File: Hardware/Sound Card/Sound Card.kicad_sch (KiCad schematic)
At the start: 35 parts, among them J1 ICSP, J2 6502 Card Edge, J3 Conn_02x08_Odd_Even, J4 PORT A, J5 3.5mm TRS, U1 ATmega328P-A, U2 74HC245, U3 74HC245, U4 74HC138, U5 AY-3-8912, U6 LM386, X1 2 MHz, Y1 16MHz

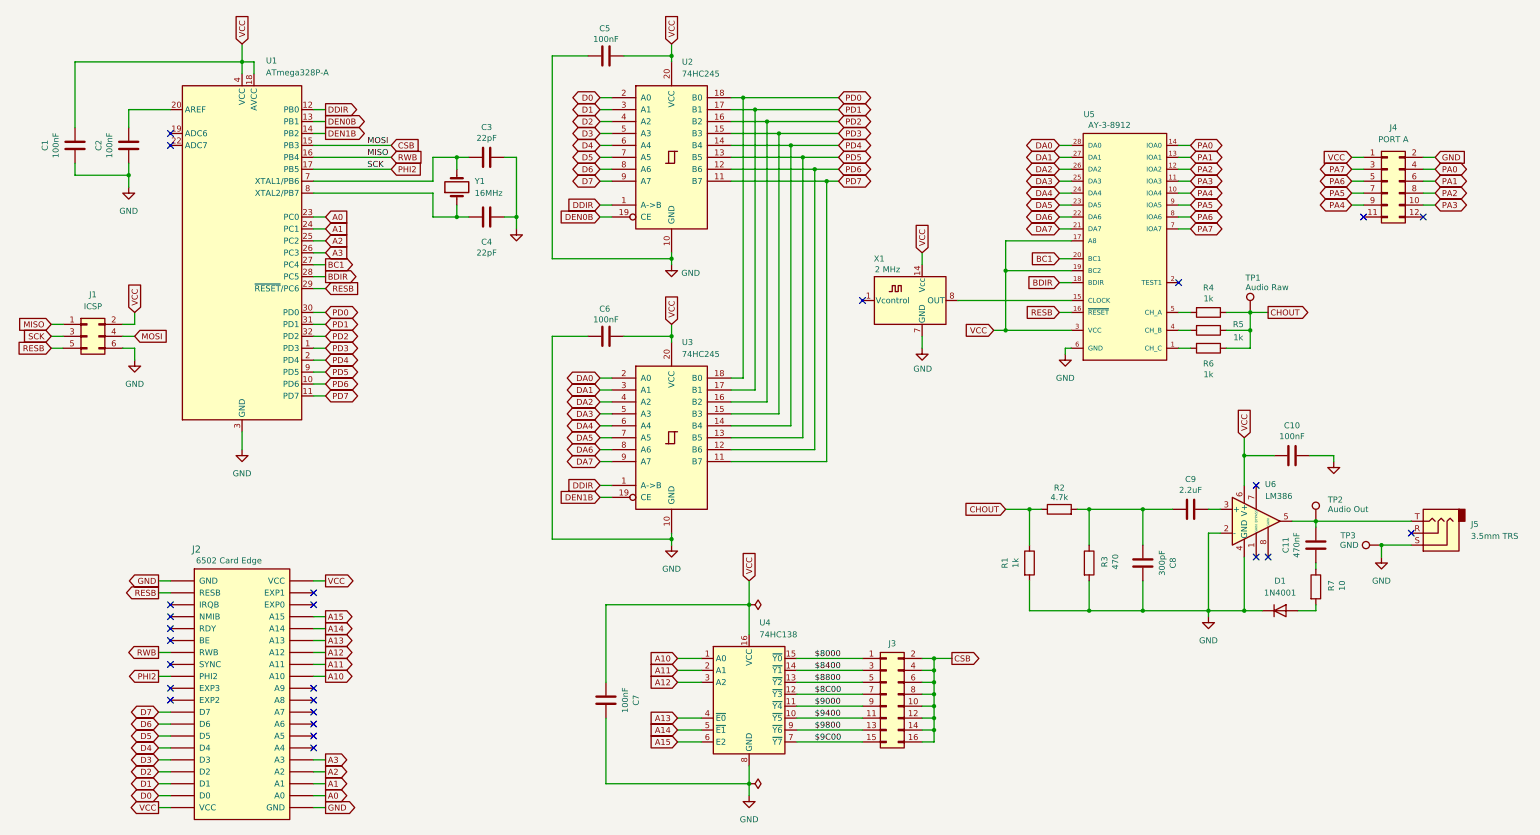
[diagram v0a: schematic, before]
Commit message: Add Wozmon
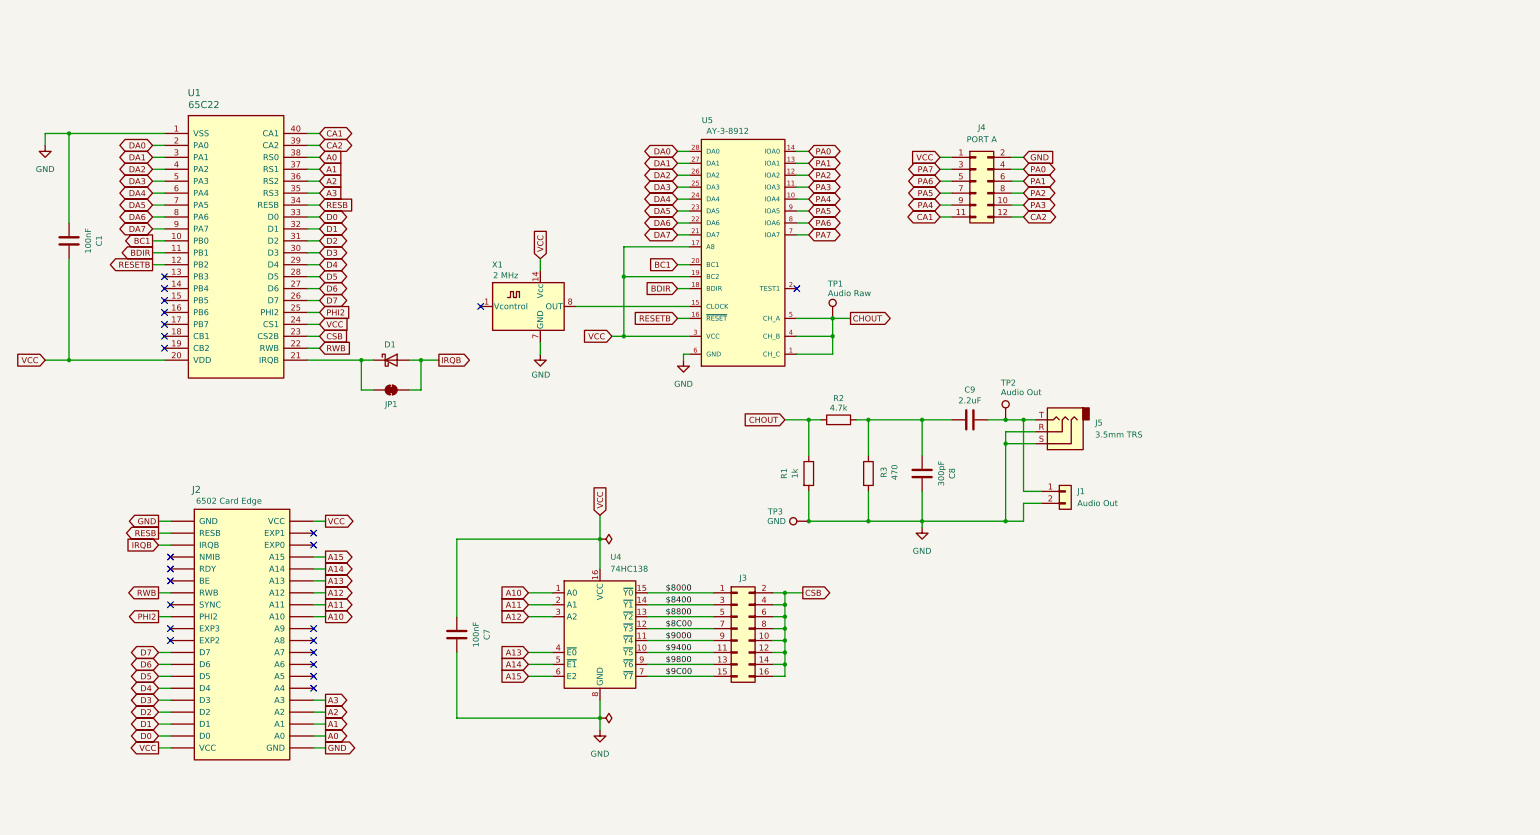
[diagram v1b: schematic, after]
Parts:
- removed C10, C2, C5, C6: 100nF, Capacitor_SMD:C_0805_2012Metric, symbol Device:C
- removed C11: 470nF, Capacitor_SMD:C_0805_2012Metric, symbol Device:C
- removed C3, C4: 22pF, Capacitor_SMD:C_0805_2012Metric, symbol Device:C
- removed D1: 1N4001, Diode_SMD:D_SMA, symbol Diode:1N4001
- removed J1: ICSP, Connector_PinHeader_2.54mm:PinHeader_2x03_P2.54mm_Vertical, symbol Connector_Generic:Conn_02x03_Odd_Even
- removed R4, R5, R6: 1k, Resistor_SMD:R_0805_2012Metric, symbol Device:R
- removed R7: 10, Resistor_SMD:R_0805_2012Metric, symbol Device:R
- removed U1: ATmega328P-A, Package_QFP:TQFP-32_7x7mm_P0.8mm, symbol MCU_Microchip_ATmega:ATmega328P-A
- removed U2, U3: 74HC245, Package_SO:SOIC-20W_7.5x12.8mm_P1.27mm, symbol 74xx:74HC245
- removed U6: LM386, Package_SO:SOP-8_3.76x4.96mm_P1.27mm, symbol Amplifier_Audio:LM386
- removed Y1: 16MHz, Crystal:Crystal_HC49-U_Vertical, symbol Device:Crystal
- added D1: D_Schottky, Diode_THT:D_DO-35_SOD27_P7.62mm_Horizontal, symbol Device:D_Schottky
- added J1: Audio Out, Connector_JST:JST_XH_B2B-XH-A_1x02_P2.50mm_Vertical, symbol Connector_Generic:Conn_01x02
- added JP1: SolderJumper_2_Bridged, Jumper:SolderJumper-2_P1.3mm_Bridged_RoundedPad1.0x1.5mm, symbol Jumper:SolderJumper_2_Bridged
- added U1: 65C22, Package_DIP:DIP-40_W15.24mm_Socket_LongPads, symbol 6502 Parts:65C22
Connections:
- net A0: now also U1.38 (RS0)
- net A1: now also U1.37 (RS1)
- net A2: now also U1.36 (RS2)
- net A3: now also U1.35 (RS3)
- net BC1: now also U1.10 (PB0)
- net BDIR: now also U1.11 (PB1)
- net CHOUT: now also U5.1 (CH_C), U5.4 (CH_B), U5.5 (CH_A)
- net CSB: now also U1.23 (CS2B)
- net D0: now also U1.33 (D0)
- net D1: now also U1.32 (D1)
- net D2: now also U1.31 (D2)
- net D3: now also U1.30 (D3)
- net D4: now also U1.29 (D4)
- net D5: now also U1.28 (D5)
- net D6: now also U1.27 (D6)
- net D7: now also U1.26 (D7)
- net DA0: now also U1.2 (PA0)
- net DA1: now also U1.3 (PA1)
- net DA2: now also U1.4 (PA2)
- net DA3: now also U1.5 (PA3)
- net DA4: now also U1.6 (PA4)
- net DA5: now also U1.7 (PA5)
- net DA6: now also U1.8 (PA6)
- net DA7: now also U1.9 (PA7)
- net GND: now also J5.R, J1.2 (Pin_2), U1.1 (VSS)
- net PHI2: now also U1.25 (PHI2)
- net RESB: now also U1.34 (RESB); no longer U5.16 (~{RESET})
- net VCC: now also U1.20 (VDD), U1.24 (CS1)
- net at C9.2: now also J5.T, TP2.1, J1.1 (Pin_1)
- net CA1: now reaches J4.11 (Pin_11)
- net CA1: now also U1.40 (CA1)
- net CA2: now reaches J4.12 (Pin_12)
- net CA2: now also U1.39 (CA2)
- net IRQB: now reaches J2.IRQB
- net IRQB: now also D1.2 (A), JP1.2 (B)
- net MISO renamed RWB
- net RWB: now also U1.22 (RWB)
- new net: D1.1 (K), JP1.1 (A), U1.21 (IRQB)
- new net RESETB: U1.12 (PB2), U5.16 (~{RESET})
- no-connect marks 25 -> 23
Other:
- moved on the sheet: C7, C8, C9, J2, J3, J4, J5, R1, R2, R3, TP1, TP2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
